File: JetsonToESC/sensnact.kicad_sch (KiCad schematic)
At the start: 13 parts, among them U2 DS18B20, U5 ACS759ECB-200B-PFF-T

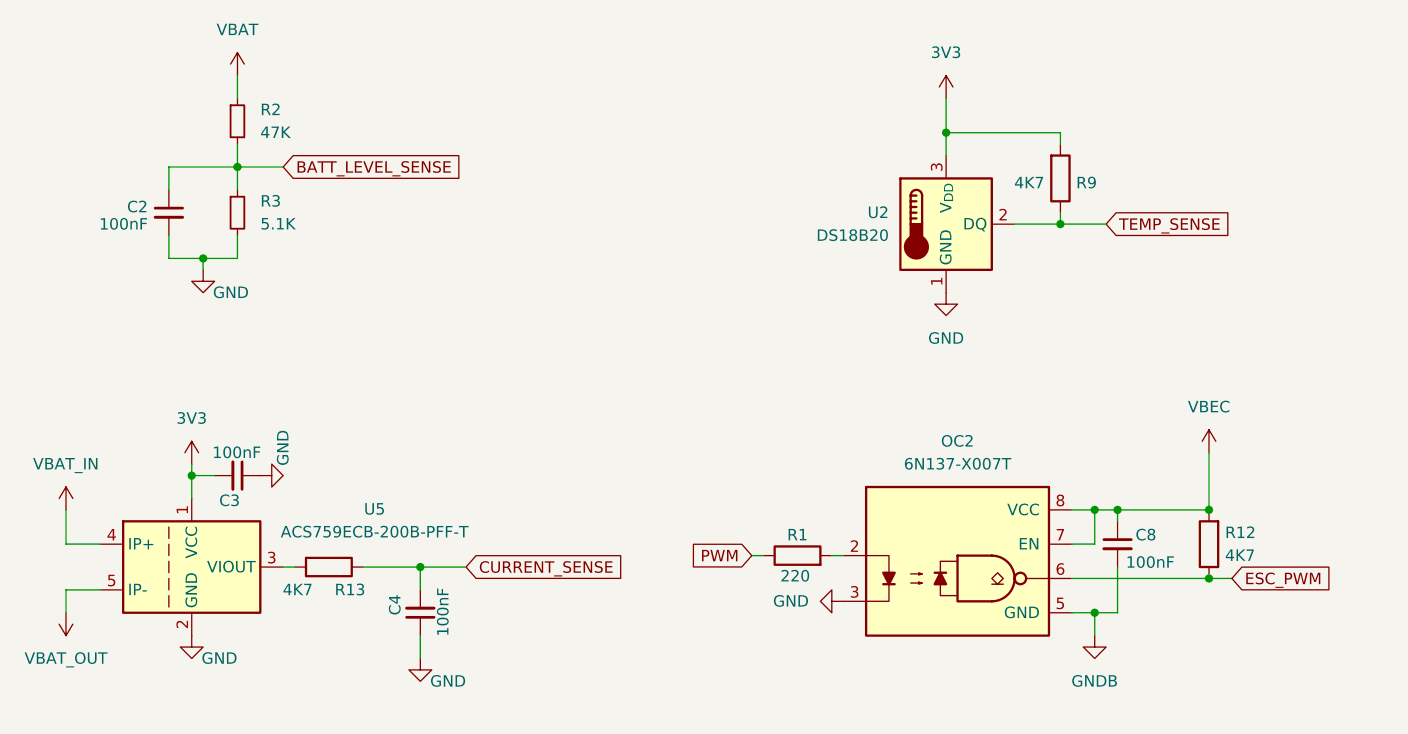
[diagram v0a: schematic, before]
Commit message: Updated for v2.0, almost complete
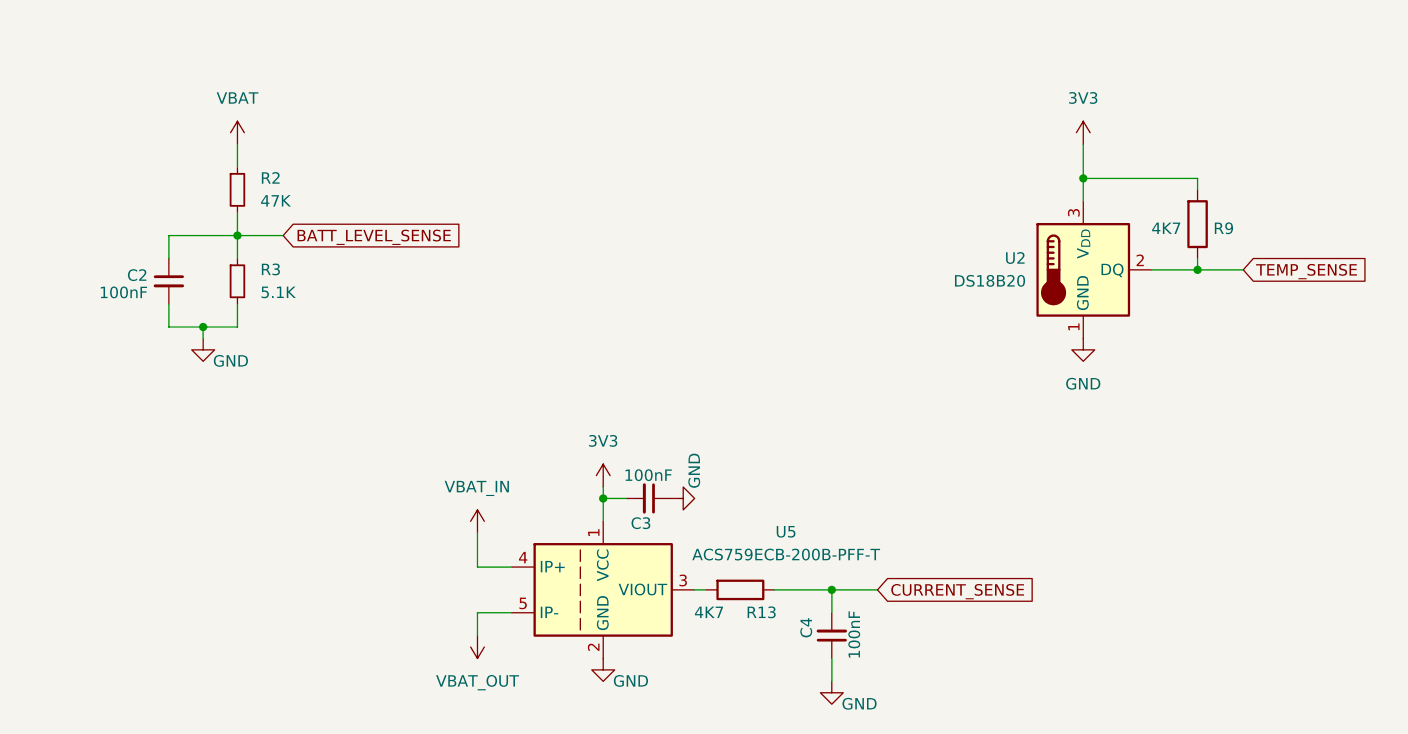
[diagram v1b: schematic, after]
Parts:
- removed C8: 100nF, Capacitor_SMD:C_0603_1608Metric, symbol Device:C_Small
- removed OC2: 6N137-X007T, PCM_Package_DIP_AKL:SMDIP-8_W9.53mm, symbol PCM_Optocoupler_Logic_AKL:6N137-X007T
- removed R1: 220, Resistor_SMD:R_0603_1608Metric, symbol Device:R
- removed R12: 4K7, Resistor_SMD:R_0603_1608Metric, symbol Device:R
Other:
- moved on the sheet: C2, C3, C4, R13, R2, R3, R9, U2, U5
